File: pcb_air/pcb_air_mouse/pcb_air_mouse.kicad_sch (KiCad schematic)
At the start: 2 parts, among them U1 MPU-6050

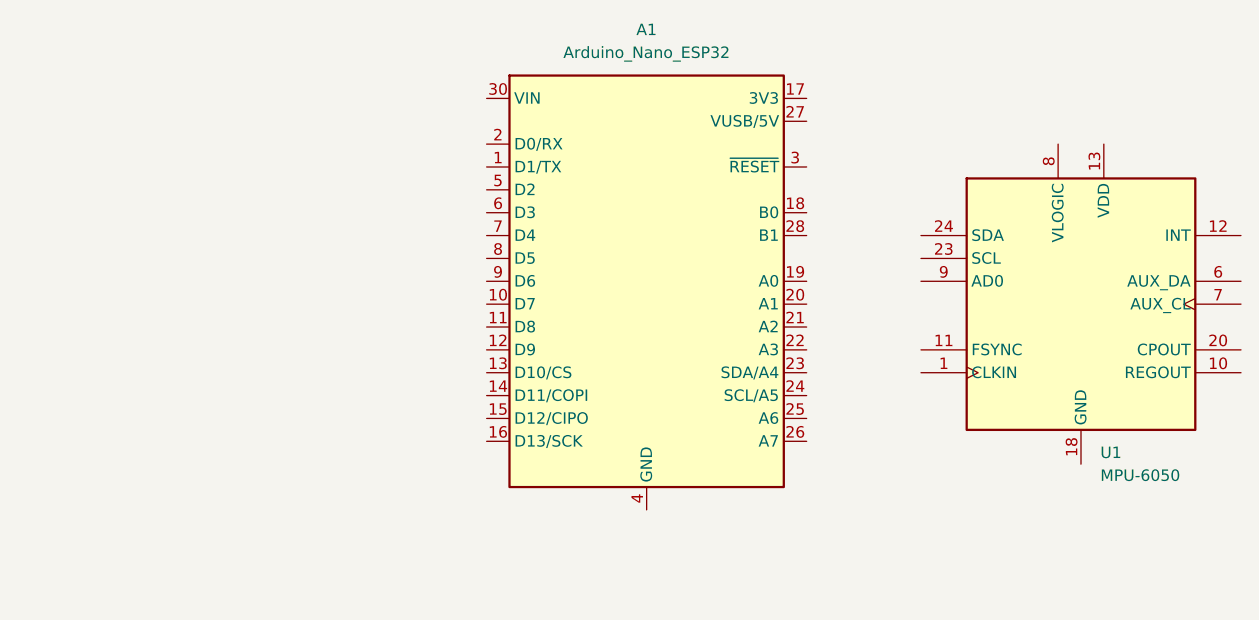
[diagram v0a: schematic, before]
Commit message: Gitpush
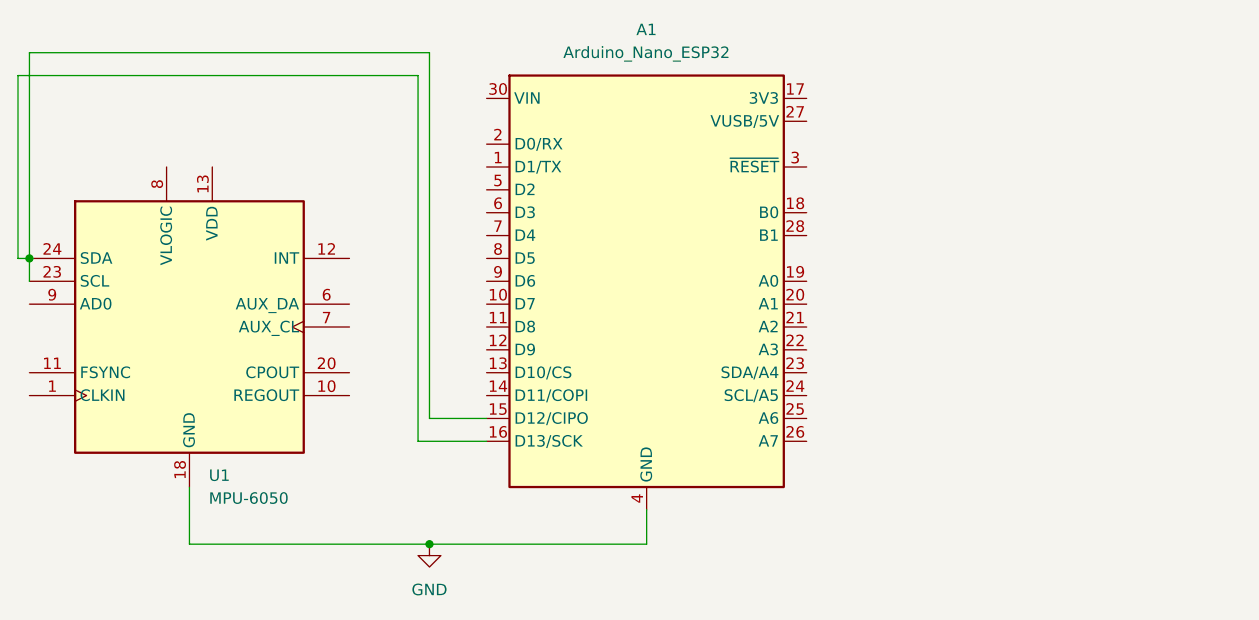
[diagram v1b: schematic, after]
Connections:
- net GND: now reaches U1.18 (GND)
- net GND: now also A1.29 (GND), A1.4 (GND)
- net at U1.23 (SCL): now also A1.15 (D12/CIPO), A1.16 (D13/SCK), U1.24 (SDA)
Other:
- moved on the sheet: U1
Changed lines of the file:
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@@
 	(generator_version "9.0")
 	(paper "A4")
+	(junction
+		(at 111.76 116.84)
+		(diameter 0)
+		(color 0 0 0 0)
+	)
+	(junction
+		(at 67.31 85.09)
+		(diameter 0)
+		(color 0 0 0 0)
+	)
+	(wire
+		(pts
+			(xy 135.89 116.84) (xy 135.89 113.03)
+		)
+		(stroke
+			(width 0)
+			(type default)
+		)
+	)
+	(wire
+		(pts
+			(xy 111.76 102.87) (xy 118.11 102.87)
+		)
+		(stroke
+			(width 0)
+			(type default)
+		)
+	)
+	(wire
+		(pts
+			(xy 85.09 110.49) (xy 85.09 116.84)
+		)
+		(stroke
+			(width 0)
+			(type default)
+		)
+	)
+	(wire
+		(pts
+			(xy 67.31 85.09) (xy 67.31 62.23)
+		)
+		(stroke
+			(width 0)
+			(type default)
+		)
+	)
+	(wire
+		(pts
+			(xy 67.31 87.63) (xy 67.31 85.09)
+		)
+		(stroke
+			(width 0)
+			(type default)
+		)
+	)
+	(wire
+		(pts
+			(xy 67.31 62.23) (xy 111.76 62.23)
+		)
+		(stroke
+			(width 0)
+			(type default)
+		)
+	)
+	(wire
+		(pts
+			(xy 85.09 116.84) (xy 111.76 116.84)
+		)
+		(stroke
+			(width 0)
+			(type default)
+		)
+	)
+	(wire
+		(pts
+			(xy 111.76 62.23) (xy 111.76 102.87)
+		)
+		(stroke
+			(width 0)
+			(type default)
+		)
+	)
+	(wire
+		(pts
+			(xy 66.04 64.77) (xy 110.49 64.77)
+		)
+		(stroke
+			(width 0)
+			(type default)
+		)
+	)
+	(wire
+		(pts
+			(xy 110.49 64.77) (xy 110.49 105.41)
+		)
+		(stroke
+			(width 0)
+			(type default)
+		)
+	)
+	(wire
+		(pts
+			(xy 111.76 116.84) (xy 135.89 116.84)
+		)
+		(stroke
+			(width 0)
+			(type default)
+		)
+	)
+	(wire
+		(pts
+			(xy 67.31 85.09) (xy 66.04 85.09)
+		)
+		(stroke
+			(width 0)
+			(type default)
+		)
+	)
+	(wire
+		(pts
+			(xy 110.49 105.41) (xy 118.11 105.41)
+		)
+		(stroke
+			(width 0)
+			(type default)
+		)
+	)
+	(wire
+		(pts
+			(xy 66.04 85.09) (xy 66.04 64.77)
+		)
+		(stroke
+			(width 0)
+			(type default)
+		)
+	)
+	(symbol
+		(lib_id "power:GND")
+		(at 111.76 116.84 0)
+		(unit 1)
+		(exclude_from_sim no)
+		(in_bom yes)
+		(on_board yes)
+		(dnp no)
+		(fields_autoplaced yes)
+		(property "Reference" "#PWR01"
+			(at 111.76 123.19 0)
+			(effects
+				(font
+					(size 1.27 1.27)
+				)
+				(hide yes)
+			)
+		)
+		(property "Value" "GND"
+			(at 111.76 121.92 0)
+			(effects
+				(font
+					(size 1.27 1.27)
+				)
+			)
+		)
+		(property "Footprint" ""
+			(at 111.76 116.84 0)
+			(effects
+				(font
+					(size 1.27 1.27)
+				)
+				(hide yes)
+			)
+		)
+		(property "Datasheet" ""
+			(at 111.76 116.84 0)
+			(effects
+				(font
+					(size 1.27 1.27)
+				)
+				(hide yes)
+			)
+		)
+		(property "Description" "Power symbol creates a global label with name \"GND\" , ground"
+			(at 111.76 116.84 0)
+			(effects
+				(font
+					(size 1.27 1.27)
+				)
+				(hide yes)
+			)
+		)
+		(pin "1"
+		)
+		(instances
+			(project ""
+				(path "/3ba0ce07-30b1-4d23-a73a-76e88b2b5e68"
+					(reference "#PWR01")
+					(unit 1)
+				)
+			)
+		)
+	)
 	(symbol
 		(lib_id "Sensor_Motion:MPU-6050")
-		(at 184.15 90.17 0)
+		(at 85.09 92.71 0)
 		(unit 1)
 		(exclude_from_sim no)
@@
 		(fields_autoplaced yes)
 		(property "Reference" "U1"
-			(at 186.2933 106.68 0)
+			(at 87.2333 109.22 0)
 			(effects
 				(font
@@
 		)
 		(property "Value" "MPU-6050"
-			(at 186.2933 109.22 0)
+			(at 87.2333 111.76 0)
 			(effects
 				(font
@@
 		)
 		(property "Footprint" "Sensor_Motion:InvenSense_QFN-24_4x4mm_P0.5mm"
-			(at 184.15 110.49 0)
+			(at 85.09 113.03 0)
 			(effects
 				(font
@@
 		)
 		(property "Datasheet" "https://invensense.tdk.com/wp-content/uploads/2015/02/MPU-6000-Datasheet1.pdf"
-			(at 184.15 93.98 0)
+			(at 85.09 96.52 0)
 			(effects
 				(font
@@
 		)
 		(property "Description" "InvenSense 6-Axis Motion Sensor, Gyroscope, Accelerometer, I2C"
-			(at 184.15 90.17 0)
-			(effects
-				(font
+			(at 85.09 92.71 0)
+			(effects
+				(font
